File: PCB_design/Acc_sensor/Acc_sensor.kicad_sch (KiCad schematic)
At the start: 45 parts, among them Q1 NMOS, Q2 NMOS, SW1 SW_SPST, SW2 SW_SPST, U1 ESP32-C3, U2 LIS2DE12, U3 DW01A, U3 MAX17263xxTE, U4 MAX30102, U5 TPS22917LDBV, U6 TPS78218DDC, U7 TLV75533PDBV

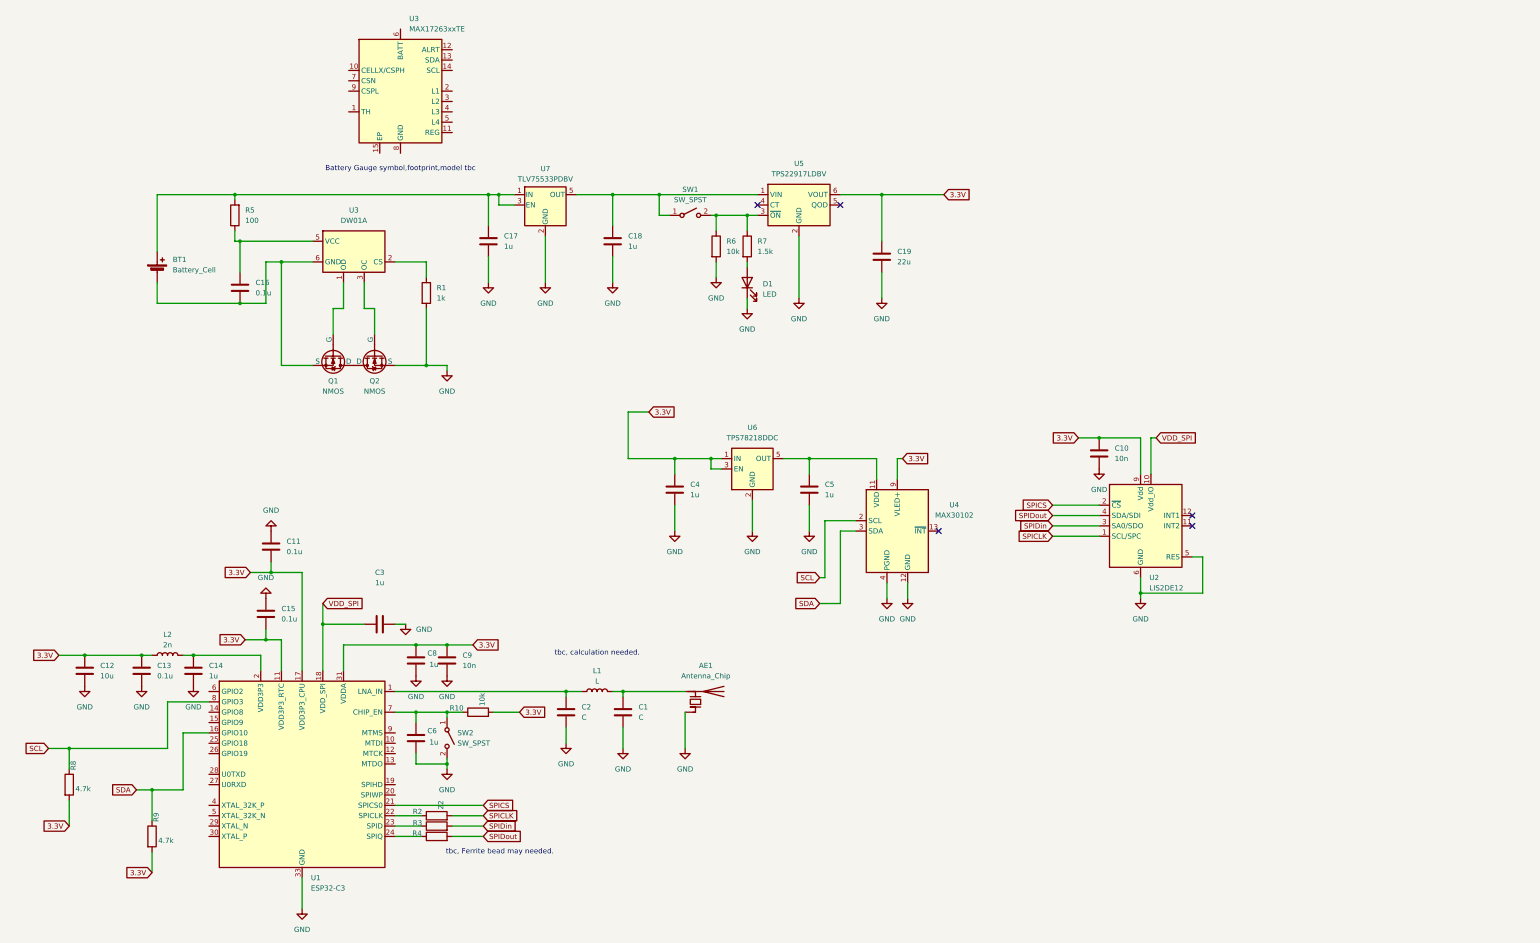
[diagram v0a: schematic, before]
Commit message: usb
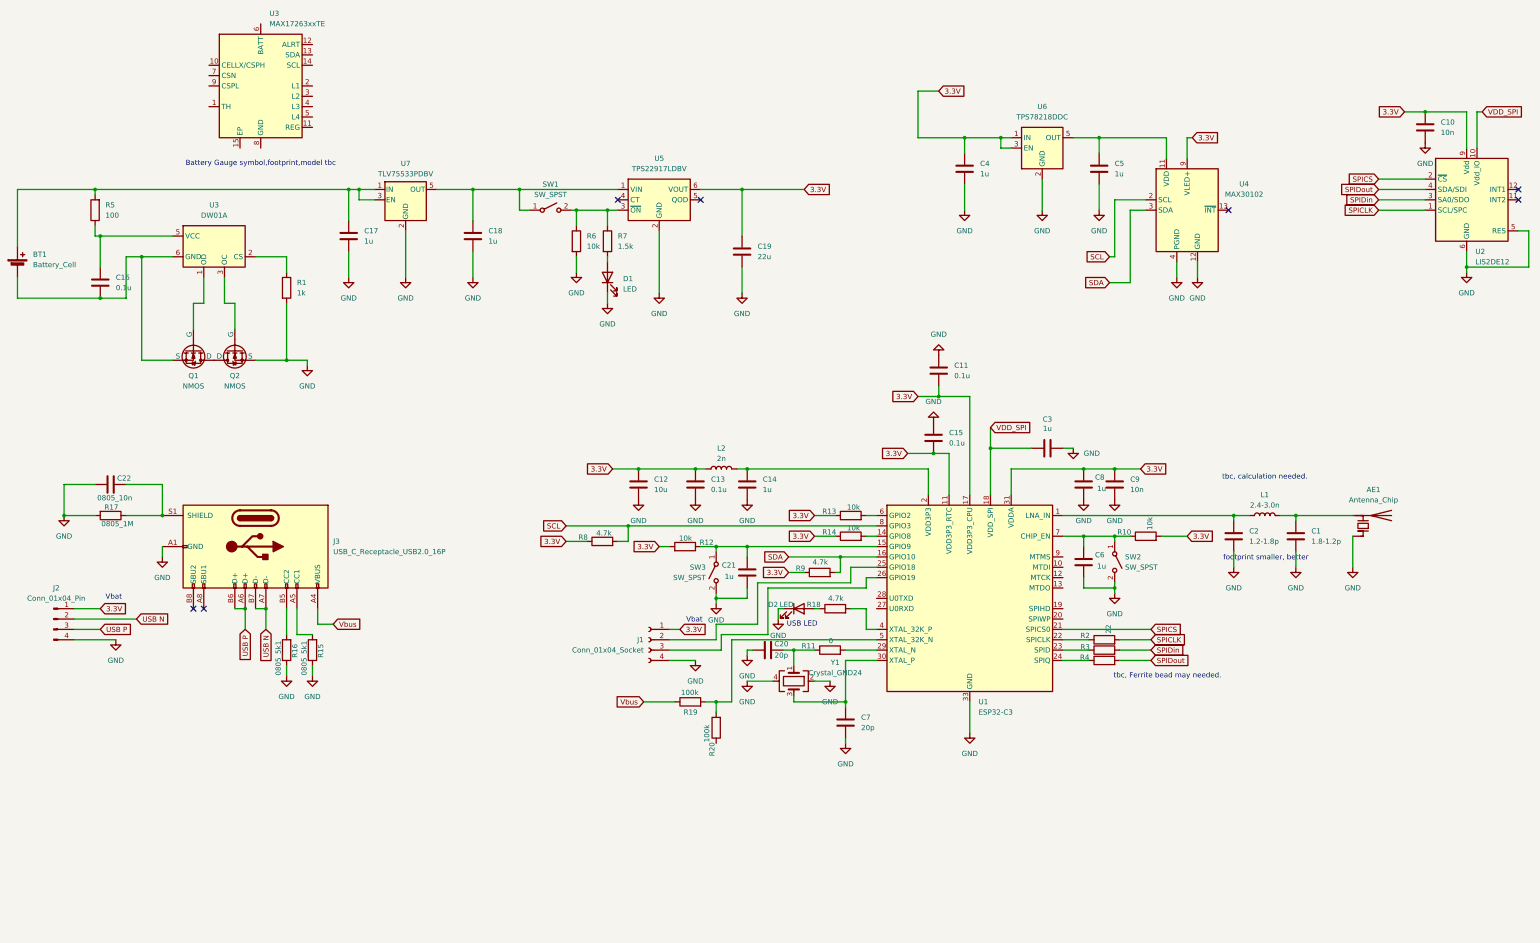
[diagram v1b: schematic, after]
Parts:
- added C20, C7: 20p, symbol Device:C
- added C21: 1u, symbol Device:C
- added C22: 0805_10n, symbol Device:C
- added D2: LED, symbol Device:LED
- added J1: Conn_01x04_Socket, symbol Connector:Conn_01x04_Socket
- added J2: Conn_01x04_Pin, symbol Connector:Conn_01x04_Pin
- added J3: USB_C_Receptacle_USB2.0_16P, symbol Connector:USB_C_Receptacle_USB2.0_16P
- added R11: 0, symbol Device:R
- added R12, R13, R14: 10k, symbol Device:R
- added R15, R16: 0805_5k1, symbol Device:R
- added R17: 0805_1M, symbol Device:R
- added R18: 4.7k, symbol Device:R
- added R19, R20: 100k, symbol Device:R
- added SW3: SW_SPST, symbol Switch:SW_SPST
- added Y1: Crystal_GND24, symbol Device:Crystal_GND24
- C1: value C -> 1.8-1.2p
- C2: value C -> 1.2-1.8p
- L1: value L -> 2.4-3.0n
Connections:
- net 3.3V: now also R8.1, R9.1, J1.1 (Pin_1), J2.1 (Pin_1), R12.2, R13.1, R14.1; no longer R8.2, R9.2
- net GND: now also C20.1, C21.2, C22.1, C7.2, D2.1 (K), J1.4 (Pin_4), J2.4 (Pin_4), J3.A1 (GND), J3.A12 (GND), J3.B1 (GND), J3.B12 (GND), R15.1, R16.1, R17.2, SW3.2 (B), Y1.2, Y1.4
- net SCL: now also R8.2; no longer R8.1
- net SDA: now also R9.2; no longer R9.1
- net at U1.14 (GPIO8): now also R14.2
- net at U1.15 (GPIO9): now also C21.1, R12.1, SW3.1 (A)
- net at U1.25 (GPIO18): now also J1.2 (Pin_2)
- net at U1.26 (GPIO19): now also J1.3 (Pin_3)
- net at U1.29 (XTAL_N): now also R11.2
- net at U1.30 (XTAL_P): now also C7.1, Y1.3
- net at U1.4 (XTAL_32K_P): now also R18.2
- net at U1.5 (XTAL_32K_N): now also R19.2, R20.2
- net at U1.6 (GPIO2): now also R13.2
- new net: C20.2, R11.1, Y1.1
- new net: C22.2, J3.S1 (SHIELD), R17.1
- new net: D2.2 (A), R18.1
- new net: J3.B5 (CC2), R16.2
- new net: J3.A5 (CC1), R15.2
- new net USB N: J2.2 (Pin_2), J3.A7 (D-), J3.B7 (D-)
- new net USB P: J2.3 (Pin_3), J3.A6 (D+), J3.B6 (D+)
- new net Vbus: J3.A4 (VBUS), J3.A9 (VBUS), J3.B4 (VBUS), J3.B9 (VBUS), R19.1
- no-connect marks 5 -> 7
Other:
- note added: "USB LED"
- note added: "Vbat"
- note added: "footprint smaller, better"
- moved on the sheet: AE1, BT1, C1, C10, C11, C12, C13, C14, C15, C16, C17, C18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
